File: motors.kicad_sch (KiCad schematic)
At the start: 17 parts, among them J10 Conn_01x04_Pin, J11 Conn_01x04_Pin, J3 Conn_02x03_Odd_Even, J4 Conn_01x04_Pin, J5 Conn_02x03_Odd_Even, J6 Conn_01x04_Pin, J7 Conn_02x03_Odd_Even, J8 Conn_01x04_Pin, J9 Conn_02x03_Odd_Even

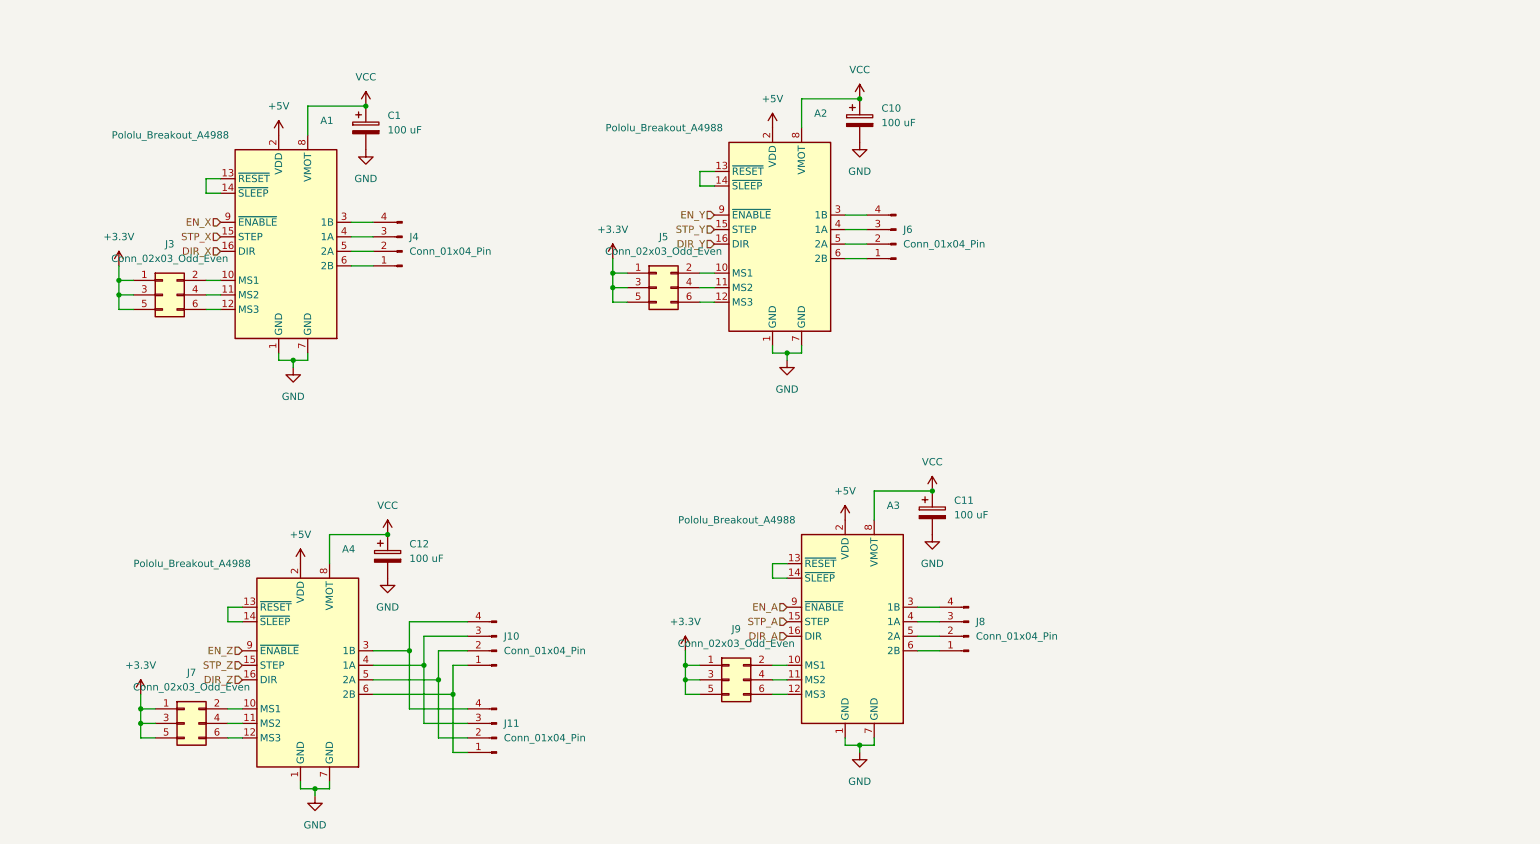
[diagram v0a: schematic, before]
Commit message: TMC2209 progress
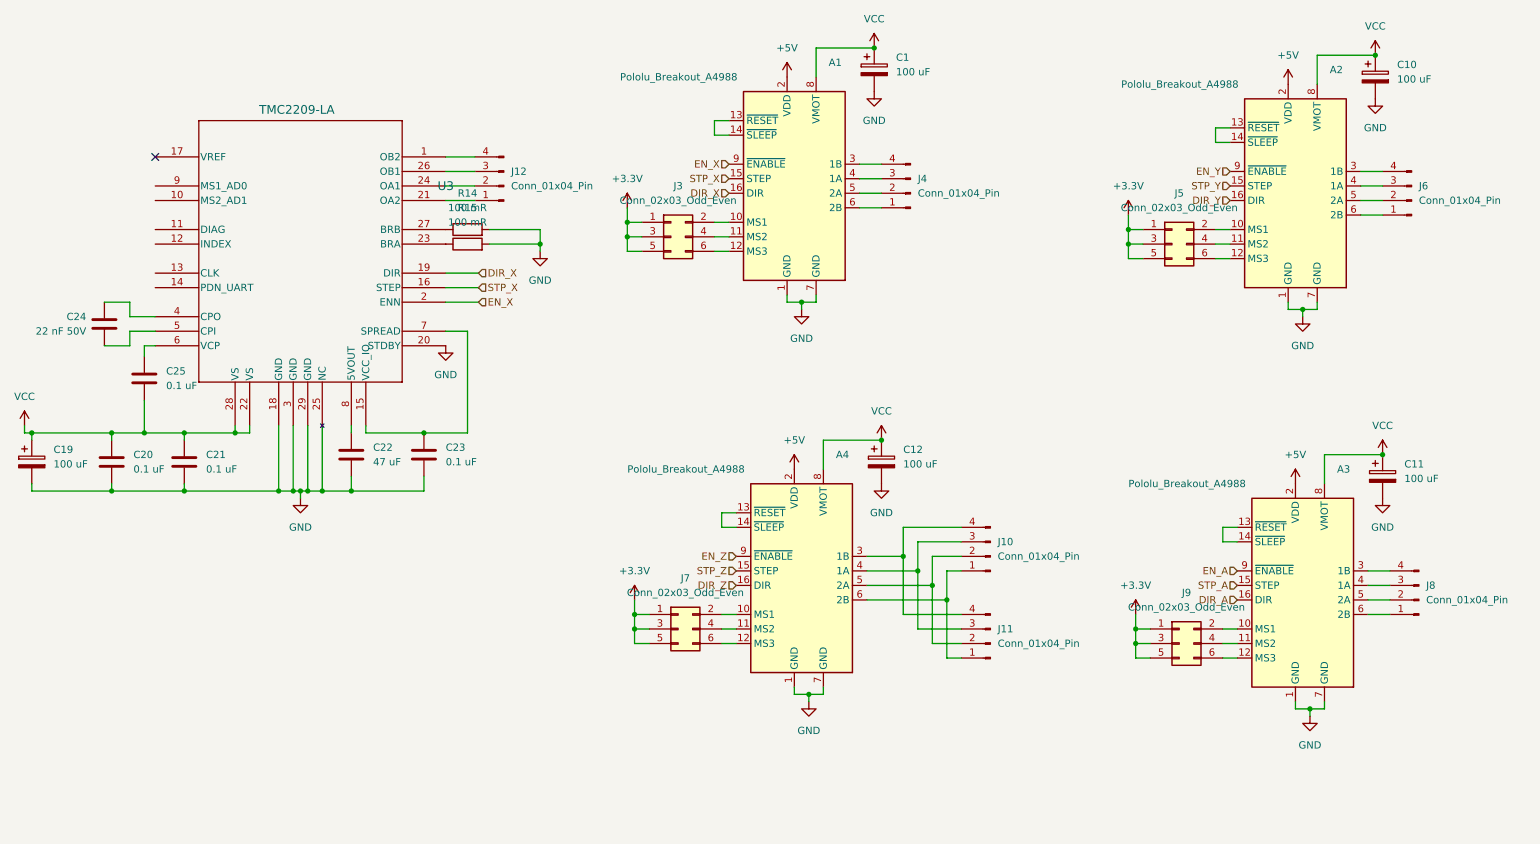
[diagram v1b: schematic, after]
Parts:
- added C19: 100 uF, Capacitor_THT:C_Disc_D3.0mm_W1.6mm_P2.50mm, symbol Device:C_Polarized
- added C20, C21, C23, C25: 0.1 uF, Capacitor_SMD:C_0603_1608Metric, symbol Device:C
- added C22: 47 uF, Capacitor_SMD:C_1206_3216Metric, symbol Device:C
- added C24: 22 nF 50V, Capacitor_SMD:C_0603_1608Metric, symbol Device:C
- added J12: Conn_01x04_Pin, Connector_JST:JST_XH_B4B-XH-A_1x04_P2.50mm_Vertical, symbol Connector:Conn_01x04_Pin
- added R14, R15: 100 mR, Resistor_SMD:R_0603_1608Metric, symbol Device:R
- added U3: TMC2209-LA, QFN28_5X5_TRI, symbol rephat-symbols:TMC2209-LA
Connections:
- net DIR_X: now also U3.19 (DIR)
- net EN_X: now also U3.2 (ENN)
- net GND: now also C19.2, C20.2, C21.2, C22.2, C23.2, R14.2, R15.2, U3.18 (GND), U3.20 (STDBY), U3.25 (NC), U3.29 (GND), U3.3 (GND)
- net STP_X: now also U3.16 (STEP)
- net VCC: now also C19.1, C20.1, C21.1, C25.1, U3.22 (VS), U3.28 (VS)
- new net: C22.1, U3.8 (5VOUT)
- new net: R15.1, U3.23 (BRA)
- new net: J12.4 (Pin_4), U3.1 (OB2)
- new net: C23.1, U3.15 (VCC_IO), U3.7 (SPREAD)
- new net: J12.1 (Pin_1), U3.21 (OA2)
- new net: J12.2 (Pin_2), U3.24 (OA1)
- new net: J12.3 (Pin_3), U3.26 (OB1)
- new net: R14.1, U3.27 (BRB)
- new net: C24.2, U3.4 (CPO)
- new net: C24.1, U3.5 (CPI)
- new net: C25.2, U3.6 (VCP)
- no-connect marks 0 -> 1
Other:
- moved on the sheet: A1, A2, A3, A4, C1, C10, C11, C12, J10, J11, J3, J4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
